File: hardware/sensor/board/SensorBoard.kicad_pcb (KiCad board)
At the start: 4 copper layers, 40 x 25 mm, 36 parts, among them J1 USB_B_Mini, J2 Conn_01x04_Male, U1 93LC56BT-I/OT, U2 FT232H, U3 74LVC2G17, U4 74LVC1G374, U5 74LVC1G04, Y1 12MHz

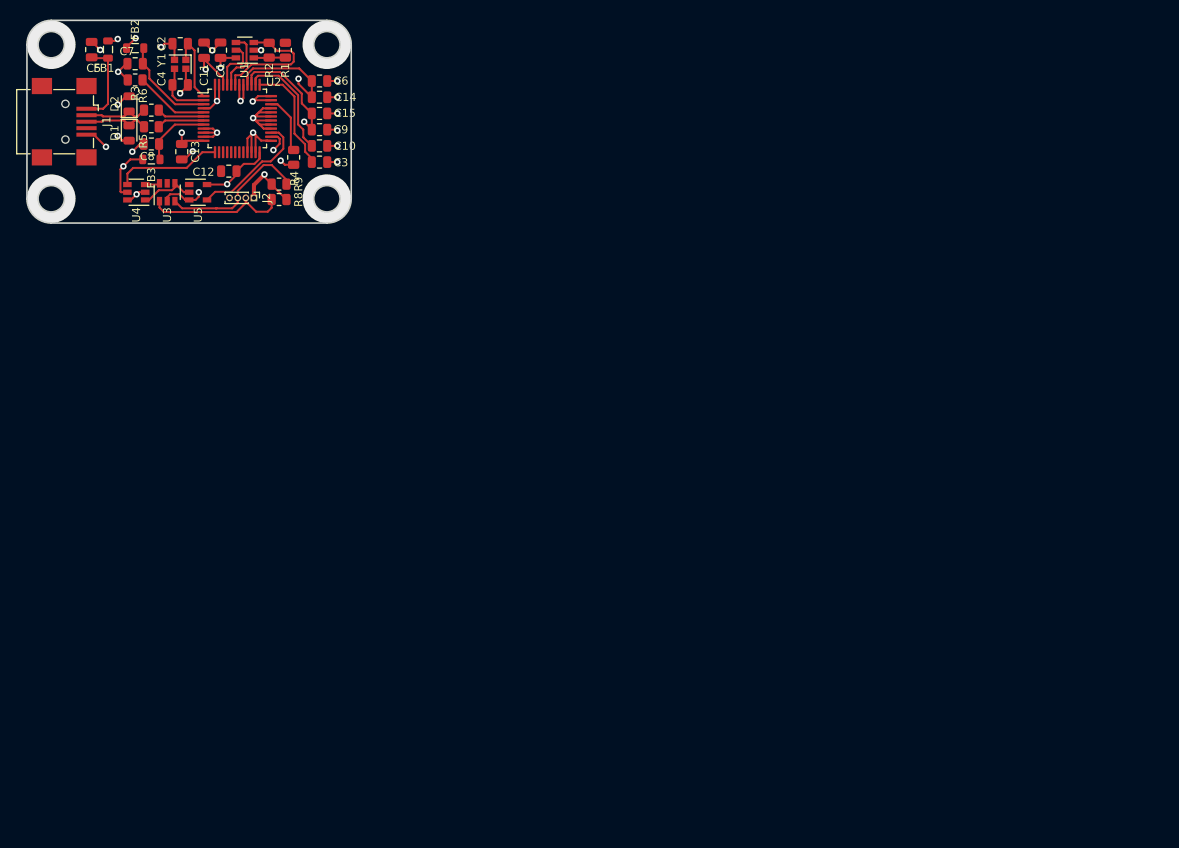
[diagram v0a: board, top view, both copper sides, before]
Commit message: Update SensorBoard.kicad_pcb
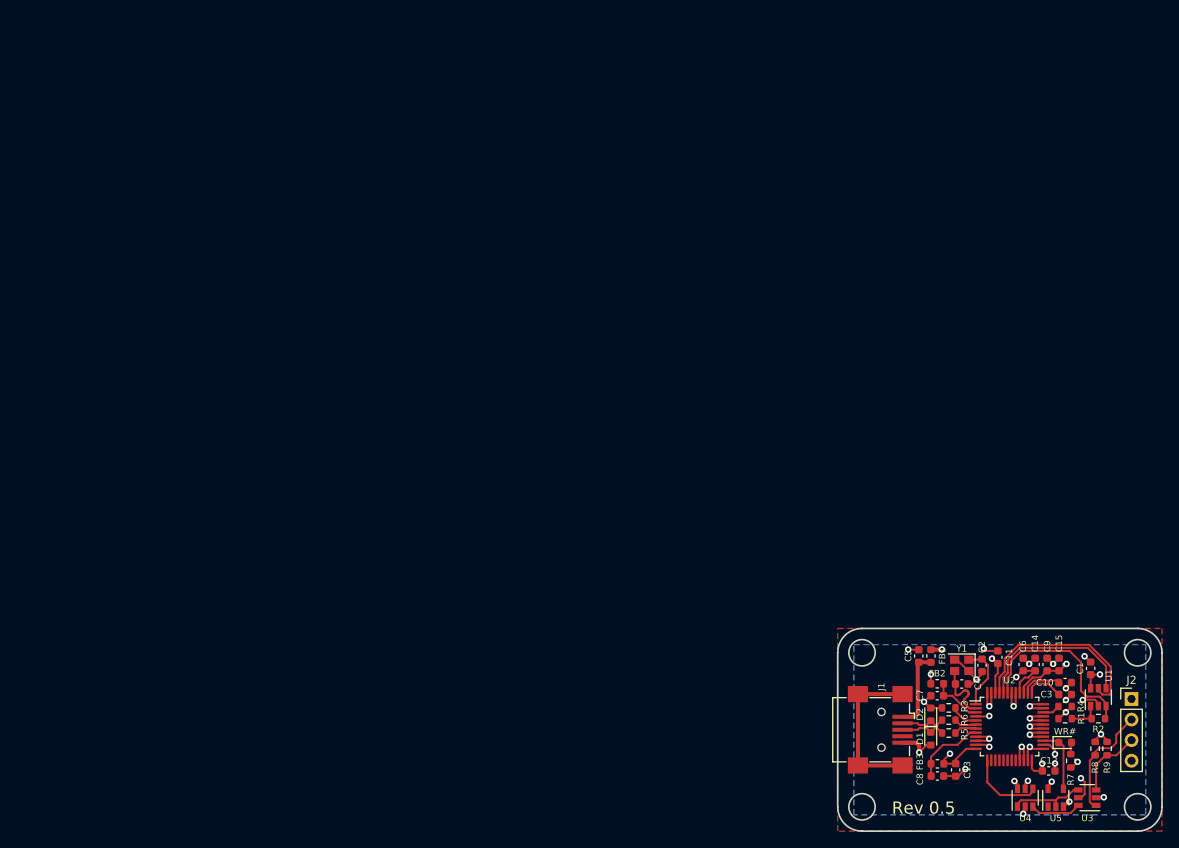
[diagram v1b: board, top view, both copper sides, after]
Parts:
- added R7: 1k, Resistor_SMD:R_0603_1608Metric, F.Cu at (128.8, 91.3)
- added WR#: LED, LED_SMD:LED_0603_1608Metric, F.Cu at (128.1, 89.1)
- C1, C3: value .1uF -> 0.1uF; footprint Capacitor_SMD:C_0805_2012Metric -> Capacitor_SMD:C_0603_1608Metric
- C10, C11, C12, C13, C14, C15, C2, C4, C5, C6, C7, C8, C9: footprint Capacitor_SMD:C_0805_2012Metric -> Capacitor_SMD:C_0603_1608Metric
- D1, D2: footprint Diode_SMD:D_0805_2012Metric -> Diode_SMD:D_0603_1608Metric
- FB1, FB2, FB3: footprint Inductor_SMD:L_0805_2012Metric -> Inductor_SMD:L_0603_1608Metric
- J2: footprint Connector_PinHeader_1.00mm:PinHeader_1x04_P1.00mm_Vertical -> Connector_PinHeader_2.54mm:PinHeader_1x04_P2.54mm_Vertical
- R1, R2, R3, R4, R5, R6, R8, R9: footprint Resistor_SMD:R_0805_2012Metric -> Resistor_SMD:R_0603_1608Metric
- Y1: footprint Crystal:Crystal_SMD_2016-4Pin_2.0x1.6mm -> Crystal:Crystal_SMD_2520-4Pin_2.5x2.0mm
- moved U3 135.8 mm to (130.8, 95.9), turned to 180 degrees
- moved U4 132.6 mm to (123.1, 95.9), turned to 90 degrees
- moved U1 132.1 mm to (132.2, 83.5), turned to 90 degrees
- moved C1 131.6 mm to (131.2, 79.9)
- moved R2 131.4 mm to (132.2, 86.1), turned to 180 degrees
- moved U5 129.5 mm to (126.9, 95.9), turned to 90 degrees
- moved R3 126.8 mm to (113.7, 84.8)
- moved R1 126.7 mm to (128.1, 86.1), turned to 0 degrees
- moved C5 126.5 mm to (110.0, 78.4)
- moved FB2 126.2 mm to (112.3, 81.8)
- moved FB1 126.1 mm to (111.5, 78.4)
- moved C7 125.9 mm to (112.3, 83.3)
- moved J1 125.5 mm to (105.4, 87.5)
- moved C12 125.3 mm to (126.0, 92.6), turned to 0 degrees
- moved C2 125.1 mm to (117.8, 79.5), turned to 270 degrees
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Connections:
- net Net-(C2-Pad1) renamed /CLK+
- net Net-(C3-Pad1) renamed /VCCA
- net Net-(C4-Pad1) renamed /CLK-
- net Net-(J2-Pad2) renamed /Phase1
- net Net-(J2-Pad3) renamed /Phase2
- net Net-(R3-Pad1) renamed /REF
- net Net-(R4-Pad1) renamed /RESET
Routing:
- net VCC3V3: track 116.4 -> 35.8 mm, vias 9 -> 11
- net VBUS: track 63.4 -> 10.4 mm
- net Net-(J1-Pad6): track 0.00 -> 19.8 mm
- net EECS: track 6.52 -> 24.8 mm
- net GND: track 87.9 -> 71.5 mm, vias 25 -> 28
- net EECLK: track 7.63 -> 20.7 mm
- net /Phase2: track 18.7 -> 8.81 mm
- net VCORE: track 14.4 -> 4.99 mm
- net /VCCA: track 13.9 -> 4.76 mm
- net EEDATA: track 15.6 -> 23.0 mm
- net WR#: track 15.2 -> 8.03 mm
- net VPHY: track 12.1 -> 6.32 mm
- net /REF: track 9.18 -> 3.38 mm
- net /RESET: track 7.26 -> 2.16 mm
- net Net-(U3-Pad6): track 1.82 -> 6.31 mm
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- added copper zone on F.Cu, net GND
- added copper zone on In1.Cu, net GND
- added copper zone on B.Cu, net VBUS
- added copper zone on In2.Cu, net VCC3V3
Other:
- net class Default: clearance 0.2 -> 0.127
- net class USB removed
- rule pad_to_mask_clearance: 0 -> 0.0508
- rule trace_clearance: 0.2 -> 0.127
- rule trace_min: 0.2 -> 0.127
- rule via_min_drill: 0.3 -> 0.254
- rule via_min_size: 0.4 -> 0.4572
- board text added: "Rev 0.5"
